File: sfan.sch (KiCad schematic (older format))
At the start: 23 parts, among them J1 Conn_01x02_Male, J2 UART, J3 SWIM, J4 Barrel_Jack, Q1 Q_NPN_EBC, Q2 SI2300, U1 STM8S003F3U, U2 AMS1117-5.0

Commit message: update
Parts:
- C3, C4: footprint (none) -> efan:C_Radial_D5.0mm_H7.0mm_P2.00mm
- J4: footprint (none) -> Connector_BarrelJack:BarrelJack_CUI_PJ-063AH_Horizontal
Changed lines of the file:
@@
 F 0 "C3" H 6218 1546 50  0000 L CNN
 F 1 "100u" H 6218 1455 50  0000 L CNN
-F 2 "" H 6138 1350 50  0001 C CNN
+F 2 "efan:C_Radial_D5.0mm_H7.0mm_P2.00mm" H 6138 1350 50  0001 C CNN
 F 3 "~" H 6100 1500 50  0001 C CNN
 	1    6100 1500
@@
 F 0 "C4" H 7118 1546 50  0000 L CNN
 F 1 "100u" H 7118 1455 50  0000 L CNN
-F 2 "" H 7038 1350 50  0001 C CNN
+F 2 "efan:C_Radial_D5.0mm_H7.0mm_P2.00mm" H 7038 1350 50  0001 C CNN
 F 3 "~" H 7000 1500 50  0001 C CNN
 	1    7000 1500
@@
 F 0 "J4" H 4821 1308 50  0000 R CNN
 F 1 "Barrel_Jack" H 4821 1399 50  0000 R CNN
-F 2 "" H 5100 1310 50  0001 C CNN
+F 2 "Connector_BarrelJack:BarrelJack_CUI_PJ-063AH_Horizontal" H 5100 1310 50  0001 C CNN
 F 3 "~" H 5100 1310 50  0001 C CNN
 	1    5050 1350

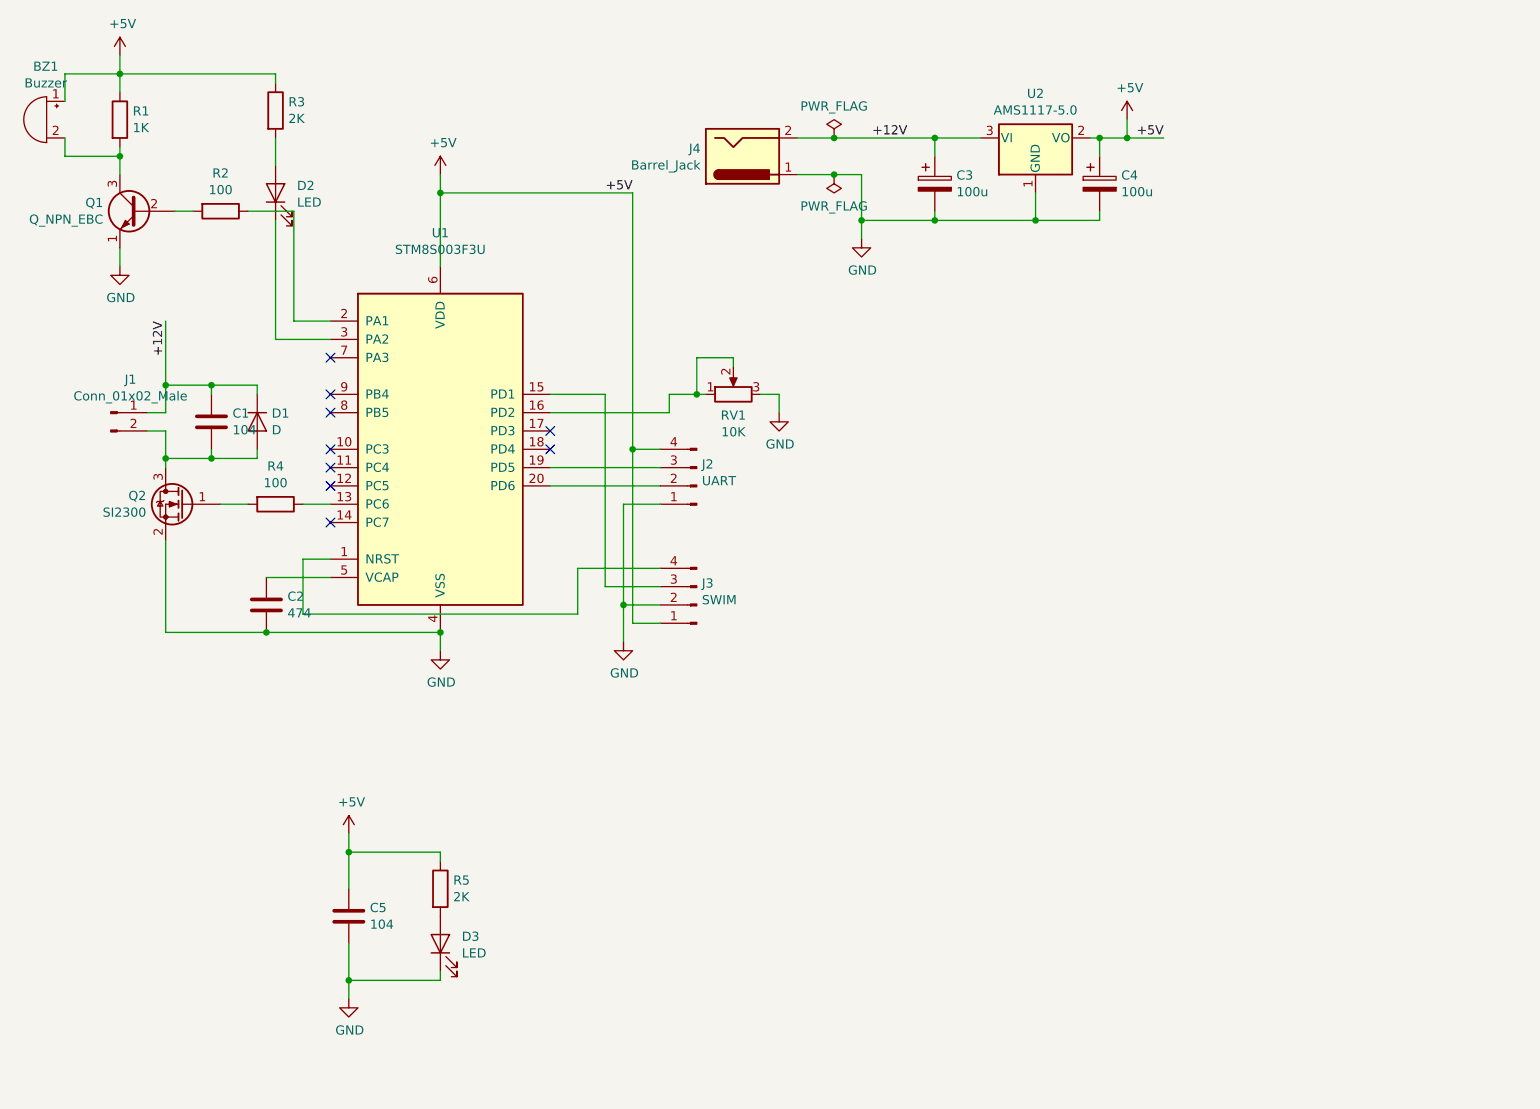
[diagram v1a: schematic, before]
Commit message: pcb layout
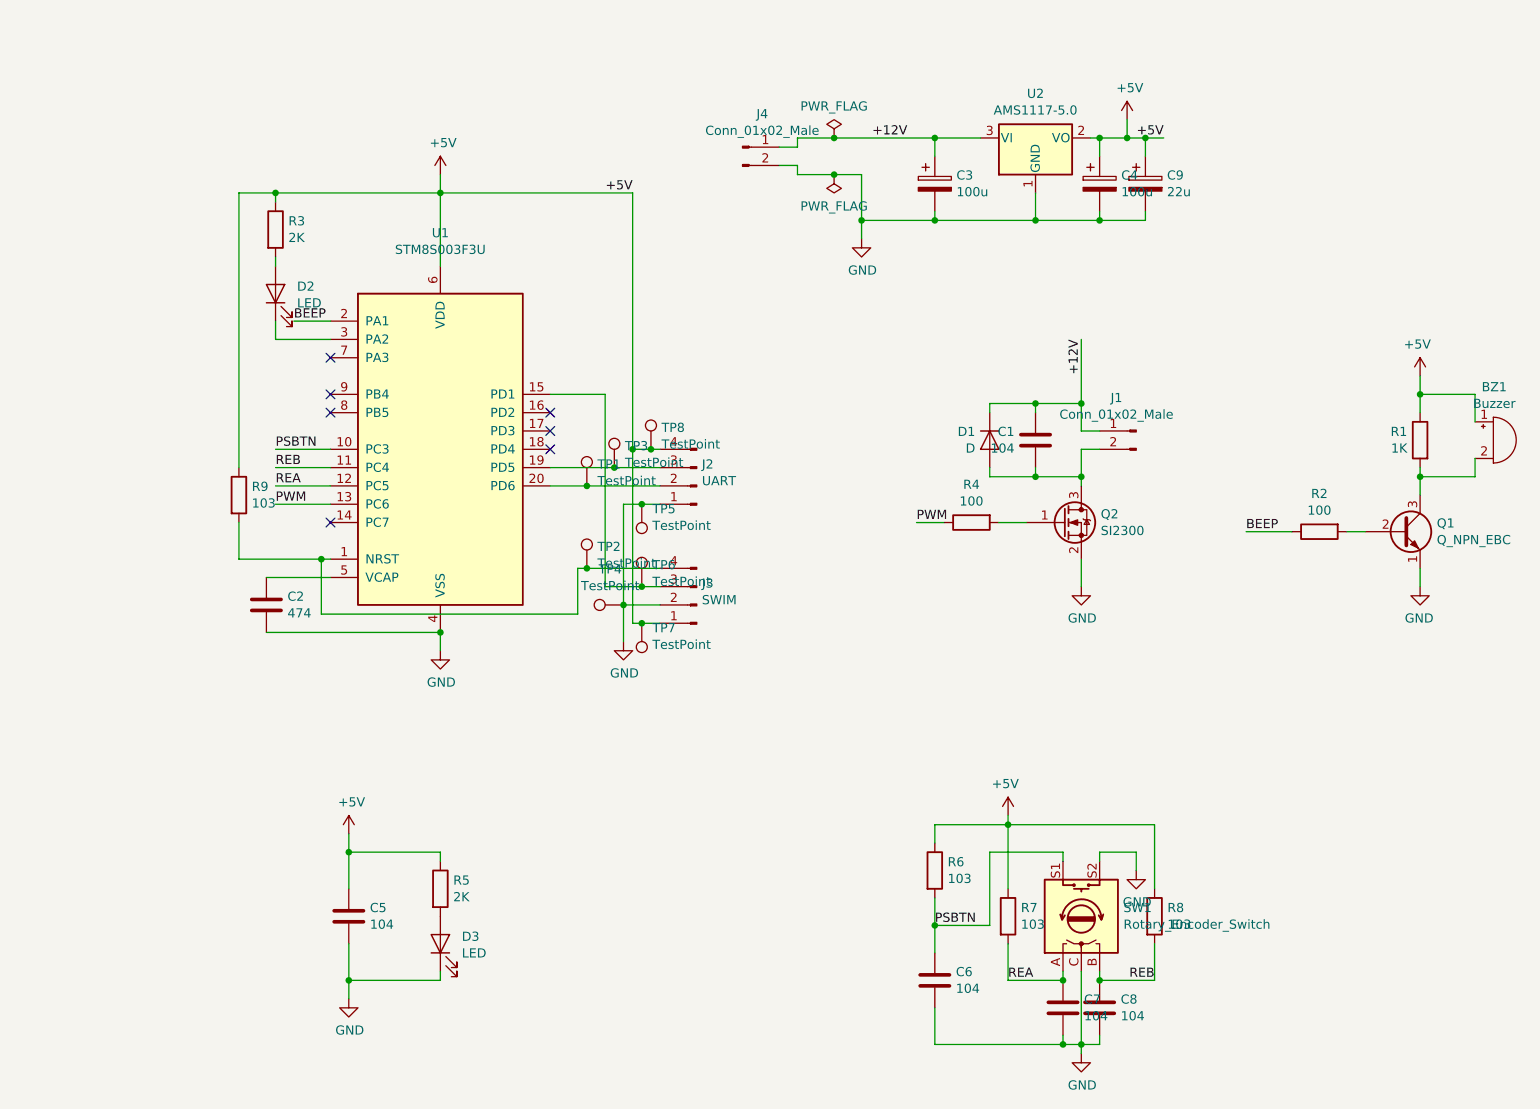
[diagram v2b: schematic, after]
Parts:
- removed J4: Barrel_Jack, Connector_BarrelJack:BarrelJack_CUI_PJ-063AH_Horizontal, symbol Connector:Barrel_Jack
- removed RV1: 10K, Connector_PinHeader_1.27mm:PinHeader_1x03_P1.27mm_Vertical, symbol Device:R_POT
- added C6, C7, C8: 104, Capacitor_SMD:C_0603_1608Metric, symbol Device:C
- added C9: 22u, Capacitor_Tantalum_SMD:CP_EIA-3216-10_Kemet-I, symbol Device:CP
- added J4: Conn_01x02_Male, Connector_PinHeader_2.54mm:PinHeader_1x02_P2.54mm_Vertical, symbol Connector:Conn_01x02_Male
- added R6, R7, R8, R9: 103, Resistor_SMD:R_0603_1608Metric, symbol Device:R
- added SW1: Rotary_Encoder_Switch, Rotary_Encoder:RotaryEncoder_Alps_EC11E-Switch_Vertical_H20mm, symbol Device:Rotary_Encoder_Switch
- added TP1, TP2, TP3, TP4, TP5, TP6, TP7, TP8: TestPoint, TestPoint:TestPoint_Pad_D1.5mm, symbol Connector:TestPoint
- C3, C4: footprint efan:C_Radial_D5.0mm_H7.0mm_P2.00mm -> EFan:C_Radial_D5.0mm_H7.0mm_P2.00mm
- D1: footprint Diode_SMD:D_0603_1608Metric -> Diode_SMD:D_SMA
- D2, D3: footprint LED_SMD:LED_0603_1608Metric -> LED_SMD:LED_0805_2012Metric
- J1: footprint Connector_PinHeader_1.27mm:PinHeader_1x02_P1.27mm_Vertical -> Connector_PinHeader_2.54mm:PinHeader_1x02_P2.54mm_Vertical
- J2, J3: footprint Connector_PinHeader_1.27mm:PinHeader_1x04_P1.27mm_Vertical -> Connector_PinHeader_2.54mm:PinHeader_1x04_P2.54mm_Vertical
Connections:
- net +12V: now also J4.1 (Pin_1)
- net +5V: now also C9.1, R6.1, R7.1, R8.1, R9.1, TP7.1, TP8.1
- net GND: now also C6.2, C7.2, C8.2, C9.2, J4.2 (Pin_2), SW1.C, SW1.S2, TP4.1, TP5.1
- net at J3.4 (Pin_4), U1.1 (NRST): now also R9.2, TP2.1
- net PSBTN: now reaches U1.10 (PC3)
- net PSBTN: now also C6.1, R6.2, SW1.S1
- net REB: now reaches U1.11 (PC4)
- net REB: now also C8.1, R8.2, SW1.B
- net REA: now reaches U1.12 (PC5)
- net REA: now also C7.1, R7.2, SW1.A
- net PWM: now reaches R4.1, U1.13 (PC6)
- net at J3.3 (Pin_3), U1.15 (PD1): now also TP6.1
- net at J2.3 (Pin_3), U1.19 (PD5): now also TP3.1
- net BEEP: now reaches R2.1, U1.2 (PA1)
- net at J2.2 (Pin_2), U1.20 (PD6): now also TP1.1
- no-connect marks 9 -> 7
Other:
- moved on the sheet: BZ1, C1, D1, D2, J1, Q1, Q2, R1, R2, R3, R4
